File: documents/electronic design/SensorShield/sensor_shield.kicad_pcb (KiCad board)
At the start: 2 copper layers, 3 parts

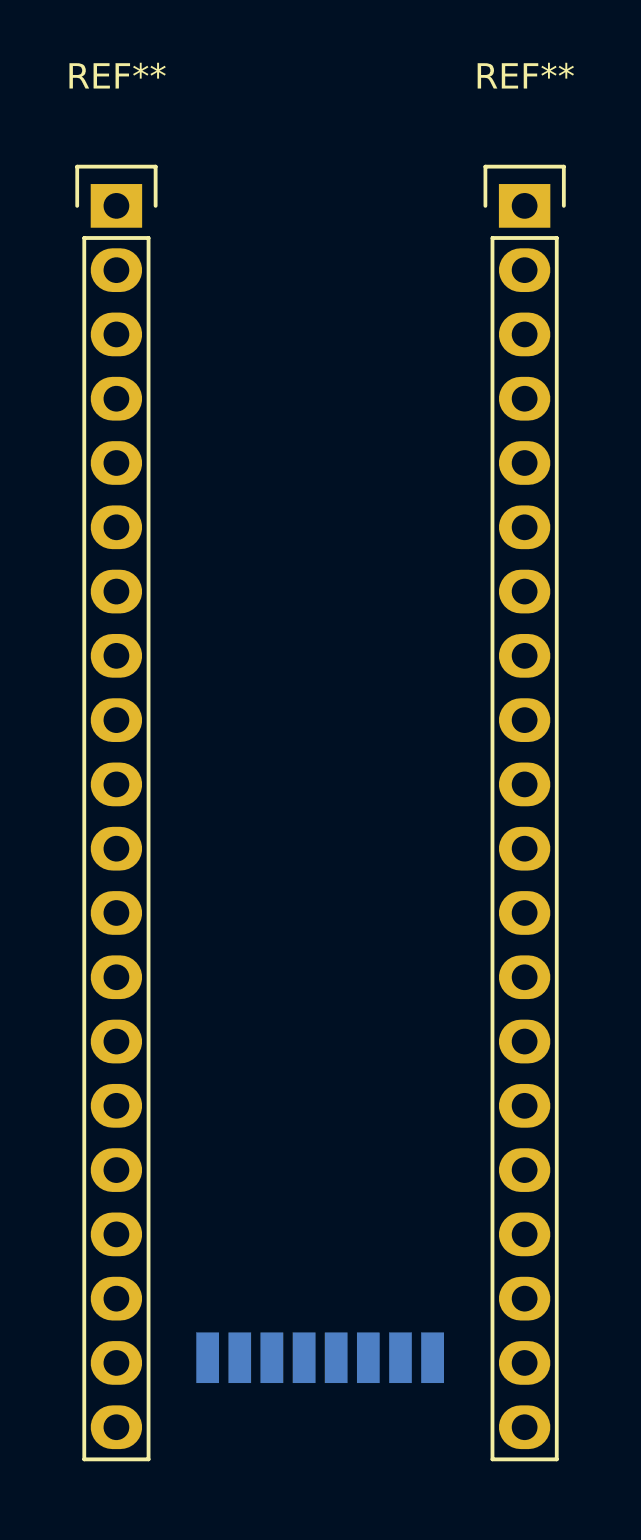
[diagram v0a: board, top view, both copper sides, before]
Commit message: update pcb draft
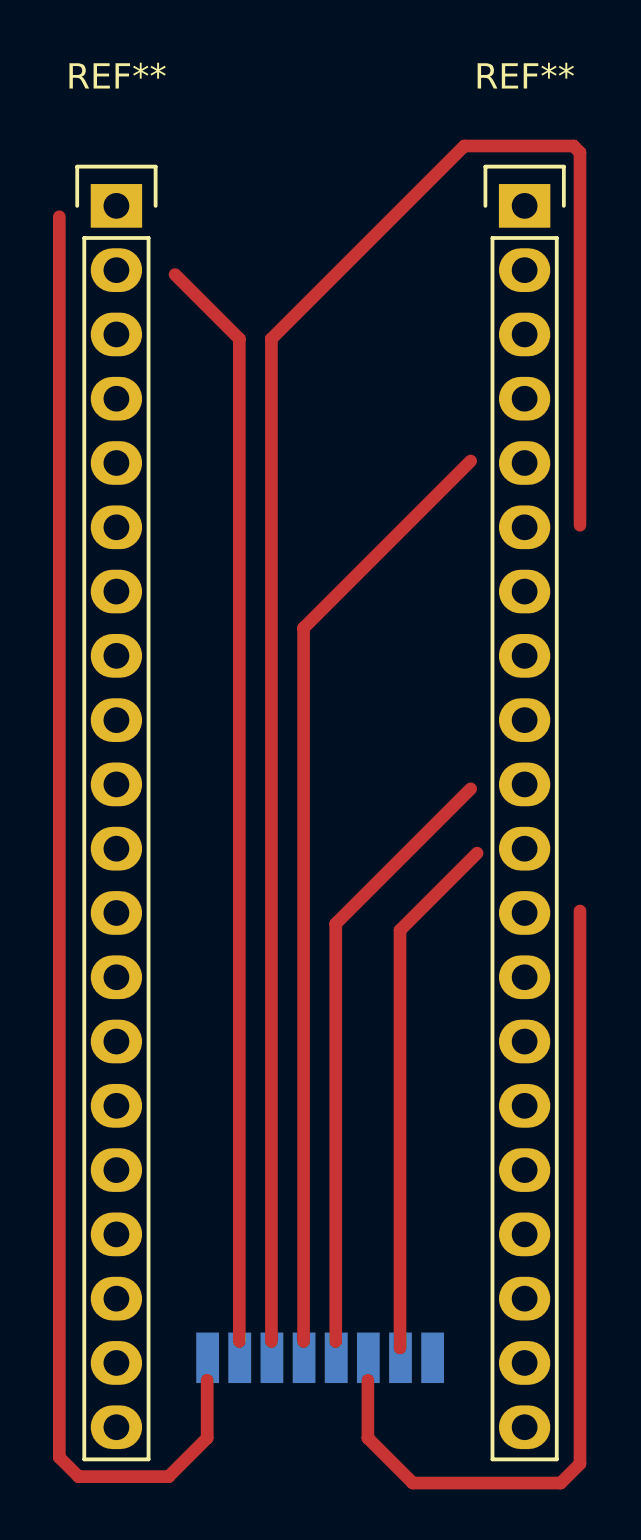
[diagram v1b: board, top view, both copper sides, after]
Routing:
- net (no net): track 0.00 -> 287.1 mm
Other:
- net class Default: trace_width 0.25 -> 0.5
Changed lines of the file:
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@@
     (links 0)
     (no_connects 0)
-    (area 0 0 0 0)
+    (area 16.650713 16.715 52.759287 81.604)
     (thickness 1.6)
     (drawings 0)
-    (tracks 0)
+    (tracks 23)
     (zones 0)
     (modules 3)
@@
   )
   (setup
-    (last_trace_width 0.25)
+    (last_trace_width 0.5)
     (trace_clearance 0.2)
     (zone_clearance 0.508)
@@
   (net_class Default "This is the default net class."
     (clearance 0.2)
-    (trace_width 0.25)
+    (trace_width 0.5)
     (via_dia 0.6)
     (via_drill 0.4)
@@
     (pad 8 smd rect (at 9.525 -12.7) (size 0.9 2) (layers B.Cu F.Paste F.Mask))
   )
+  (segment (start 44.958 72.644) (end 44.958 50.8) (width 0.5) (layer F.Cu) (net 0))
+  (segment (start 44.196 73.406) (end 44.958 72.644) (width 0.5) (layer F.Cu) (net 0))
+  (segment (start 38.354 73.406) (end 44.196 73.406) (width 0.5) (layer F.Cu) (net 0))
+  (segment (start 36.576 71.628) (end 38.354 73.406) (width 0.5) (layer F.Cu) (net 0))
+  (segment (start 36.576 69.342) (end 36.576 71.628) (width 0.5) (layer F.Cu) (net 0))
+  (segment (start 37.846 51.562) (end 40.894 48.514) (width 0.5) (layer F.Cu) (net 0))
+  (segment (start 37.846 68.072) (end 37.846 51.562) (width 0.5) (layer F.Cu) (net 0))
+  (segment (start 35.306 51.308) (end 40.64 45.974) (width 0.5) (layer F.Cu) (net 0))
+  (segment (start 35.306 67.818) (end 35.306 51.308) (width 0.5) (layer F.Cu) (net 0))
+  (segment (start 34.036 39.624) (end 40.64 33.02) (width 0.5) (layer F.Cu) (net 0))
+  (segment (start 34.036 67.818) (end 34.036 39.624) (width 0.5) (layer F.Cu) (net 0))
+  (segment (start 44.958 20.828) (end 44.958 35.56) (width 0.5) (layer F.Cu) (net 0))
+  (segment (start 44.704 20.574) (end 44.958 20.828) (width 0.5) (layer F.Cu) (net 0))
+  (segment (start 40.386 20.574) (end 44.704 20.574) (width 0.5) (layer F.Cu) (net 0))
+  (segment (start 32.766 28.194) (end 40.386 20.574) (width 0.5) (layer F.Cu) (net 0))
+  (segment (start 32.766 67.818) (end 32.766 28.194) (width 0.5) (layer F.Cu) (net 0))
+  (segment (start 31.496 28.194) (end 28.956 25.654) (width 0.5) (layer F.Cu) (net 0))
+  (segment (start 31.496 67.818) (end 31.496 28.194) (width 0.5) (layer F.Cu) (net 0))
+  (segment (start 24.384 72.39) (end 24.384 23.368) (width 0.5) (layer F.Cu) (net 0))
+  (segment (start 25.146 73.152) (end 24.384 72.39) (width 0.5) (layer F.Cu) (net 0))
+  (segment (start 28.702 73.152) (end 25.146 73.152) (width 0.5) (layer F.Cu) (net 0))
+  (segment (start 30.226 71.628) (end 28.702 73.152) (width 0.5) (layer F.Cu) (net 0))
+  (segment (start 30.226 69.342) (end 30.226 71.628) (width 0.5) (layer F.Cu) (net 0))
 )

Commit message: update pcb draft
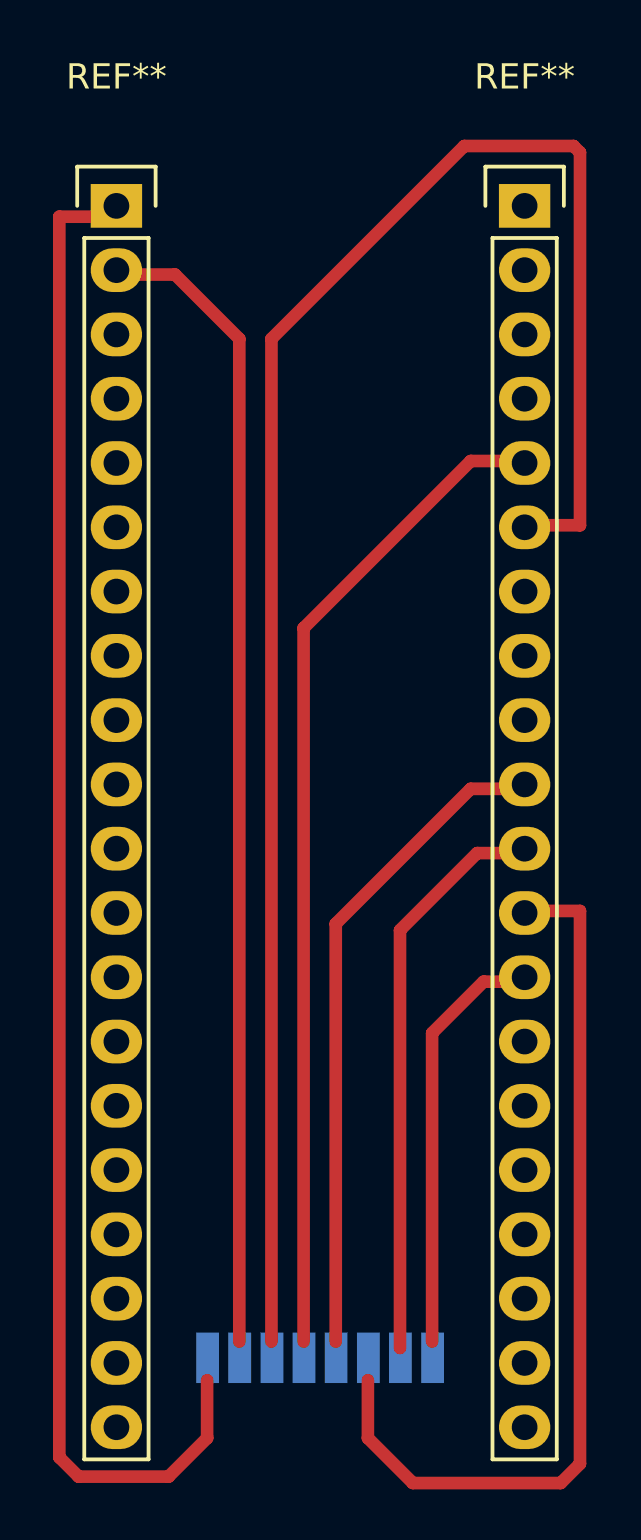
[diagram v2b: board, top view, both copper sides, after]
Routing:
- net (no net): track 287.1 -> 319.4 mm
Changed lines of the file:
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@@
     (links 0)
     (no_connects 0)
-    (area 16.650713 16.715 52.759287 81.604)
+    (area 18.174713 16.44 54.283287 81.179)
     (thickness 1.6)
     (drawings 0)
-    (tracks 23)
+    (tracks 41)
     (zones 0)
     (modules 3)
@@
       (drillshape 1)
       (scaleselection 1)
-      (outputdirectory ""))
+      (outputdirectory shield_mirror))
   )
   (net 0 "")
@@
     (pad 8 smd rect (at 9.525 -12.7) (size 0.9 2) (layers B.Cu F.Paste F.Mask))
   )
+  (segment (start 26.212 23.368) (end 24.384 23.368) (width 0.5) (layer F.Cu) (net 0))
+  (segment (start 30.226 71.628) (end 30.226 69.342) (width 0.5) (layer F.Cu) (net 0))
+  (segment (start 30.226 71.628) (end 28.702 73.152) (width 0.5) (layer F.Cu) (net 0))
+  (segment (start 28.702 73.152) (end 25.146 73.152) (width 0.5) (layer F.Cu) (net 0))
+  (segment (start 25.146 73.152) (end 24.384 72.39) (width 0.5) (layer F.Cu) (net 0))
+  (segment (start 24.384 72.39) (end 24.384 23.368) (width 0.5) (layer F.Cu) (net 0))
+  (segment (start 26.212 23.368) (end 26.64 22.94) (width 0.5) (layer F.Cu) (net 0))
+  (segment (start 26.814 25.654) (end 28.956 25.654) (width 0.5) (layer F.Cu) (net 0))
+  (segment (start 31.496 28.194) (end 31.496 67.818) (width 0.5) (layer F.Cu) (net 0))
+  (segment (start 31.496 28.194) (end 28.956 25.654) (width 0.5) (layer F.Cu) (net 0))
+  (segment (start 26.814 25.654) (end 26.64 25.48) (width 0.5) (layer F.Cu) (net 0))
+  (segment (start 42.69 33.02) (end 40.64 33.02) (width 0.5) (layer F.Cu) (net 0))
+  (segment (start 34.036 39.624) (end 34.036 67.818) (width 0.5) (layer F.Cu) (net 0))
+  (segment (start 34.036 39.624) (end 40.64 33.02) (width 0.5) (layer F.Cu) (net 0))
+  (segment (start 42.69 33.02) (end 42.77 33.1) (width 0.5) (layer F.Cu) (net 0))
+  (segment (start 42.85 35.56) (end 44.958 35.56) (width 0.5) (layer F.Cu) (net 0))
+  (segment (start 32.766 28.194) (end 32.766 67.818) (width 0.5) (layer F.Cu) (net 0))
+  (segment (start 32.766 28.194) (end 40.386 20.574) (width 0.5) (layer F.Cu) (net 0))
+  (segment (start 40.386 20.574) (end 44.704 20.574) (width 0.5) (layer F.Cu) (net 0))
+  (segment (start 44.704 20.574) (end 44.958 20.828) (width 0.5) (layer F.Cu) (net 0))
+  (segment (start 44.958 20.828) (end 44.958 35.56) (width 0.5) (layer F.Cu) (net 0))
+  (segment (start 42.85 35.56) (end 42.77 35.64) (width 0.5) (layer F.Cu) (net 0))
+  (segment (start 42.596 45.974) (end 40.64 45.974) (width 0.5) (layer F.Cu) (net 0))
+  (segment (start 35.306 51.308) (end 35.306 67.818) (width 0.5) (layer F.Cu) (net 0))
+  (segment (start 35.306 51.308) (end 40.64 45.974) (width 0.5) (layer F.Cu) (net 0))
+  (segment (start 42.596 45.974) (end 42.77 45.8) (width 0.5) (layer F.Cu) (net 0))
+  (segment (start 42.85 50.8) (end 44.958 50.8) (width 0.5) (layer F.Cu) (net 0))
+  (segment (start 36.576 71.628) (end 36.576 69.342) (width 0.5) (layer F.Cu) (net 0))
+  (segment (start 36.576 71.628) (end 38.354 73.406) (width 0.5) (layer F.Cu) (net 0))
+  (segment (start 38.354 73.406) (end 44.196 73.406) (width 0.5) (layer F.Cu) (net 0))
+  (segment (start 44.196 73.406) (end 44.958 72.644) (width 0.5) (layer F.Cu) (net 0))
   (segment (start 44.958 72.644) (end 44.958 50.8) (width 0.5) (layer F.Cu) (net 0))
-  (segment (start 44.196 73.406) (end 44.958 72.644) (width 0.5) (layer F.Cu) (net 0))
-  (segment (start 38.354 73.406) (end 44.196 73.406) (width 0.5) (layer F.Cu) (net 0))
-  (segment (start 36.576 71.628) (end 38.354 73.406) (width 0.5) (layer F.Cu) (net 0))
-  (segment (start 36.576 69.342) (end 36.576 71.628) (width 0.5) (layer F.Cu) (net 0))
+  (segment (start 42.85 50.8) (end 42.77 50.88) (width 0.5) (layer F.Cu) (net 0))
+  (segment (start 42.596 48.514) (end 40.894 48.514) (width 0.5) (layer F.Cu) (net 0))
+  (segment (start 37.846 51.562) (end 37.846 68.072) (width 0.5) (layer F.Cu) (net 0))
   (segment (start 37.846 51.562) (end 40.894 48.514) (width 0.5) (layer F.Cu) (net 0))
-  (segment (start 37.846 68.072) (end 37.846 51.562) (width 0.5) (layer F.Cu) (net 0))
-  (segment (start 35.306 51.308) (end 40.64 45.974) (width 0.5) (layer F.Cu) (net 0))
-  (segment (start 35.306 67.818) (end 35.306 51.308) (width 0.5) (layer F.Cu) (net 0))
-  (segment (start 34.036 39.624) (end 40.64 33.02) (width 0.5) (layer F.Cu) (net 0))
-  (segment (start 34.036 67.818) (end 34.036 39.624) (width 0.5) (layer F.Cu) (net 0))
-  (segment (start 44.958 20.828) (end 44.958 35.56) (width 0.5) (layer F.Cu) (net 0))
-  (segment (start 44.704 20.574) (end 44.958 20.828) (width 0.5) (layer F.Cu) (net 0))
-  (segment (start 40.386 20.574) (end 44.704 20.574) (width 0.5) (layer F.Cu) (net 0))
-  (segment (start 32.766 28.194) (end 40.386 20.574) (width 0.5) (layer F.Cu) (net 0))
-  (segment (start 32.766 67.818) (end 32.766 28.194) (width 0.5) (layer F.Cu) (net 0))
-  (segment (start 31.496 28.194) (end 28.956 25.654) (width 0.5) (layer F.Cu) (net 0))
-  (segment (start 31.496 67.818) (end 31.496 28.194) (width 0.5) (layer F.Cu) (net 0))
-  (segment (start 24.384 72.39) (end 24.384 23.368) (width 0.5) (layer F.Cu) (net 0))
-  (segment (start 25.146 73.152) (end 24.384 72.39) (width 0.5) (layer F.Cu) (net 0))
-  (segment (start 28.702 73.152) (end 25.146 73.152) (width 0.5) (layer F.Cu) (net 0))
-  (segment (start 30.226 71.628) (end 28.702 73.152) (width 0.5) (layer F.Cu) (net 0))
-  (segment (start 30.226 69.342) (end 30.226 71.628) (width 0.5) (layer F.Cu) (net 0))
+  (segment (start 42.596 48.514) (end 42.77 48.34) (width 0.5) (layer F.Cu) (net 0))
+  (segment (start 42.596 53.594) (end 41.148 53.594) (width 0.5) (layer F.Cu) (net 0))
+  (segment (start 39.116 55.626) (end 39.116 67.818) (width 0.5) (layer F.Cu) (net 0))
+  (segment (start 39.116 55.626) (end 41.148 53.594) (width 0.5) (layer F.Cu) (net 0))
+  (segment (start 42.596 53.594) (end 42.77 53.42) (width 0.5) (layer F.Cu) (net 0))
 )
